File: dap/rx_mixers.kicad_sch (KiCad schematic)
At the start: 2 parts, among them U7 SN74CBT3253, U8 SN74CBT3253

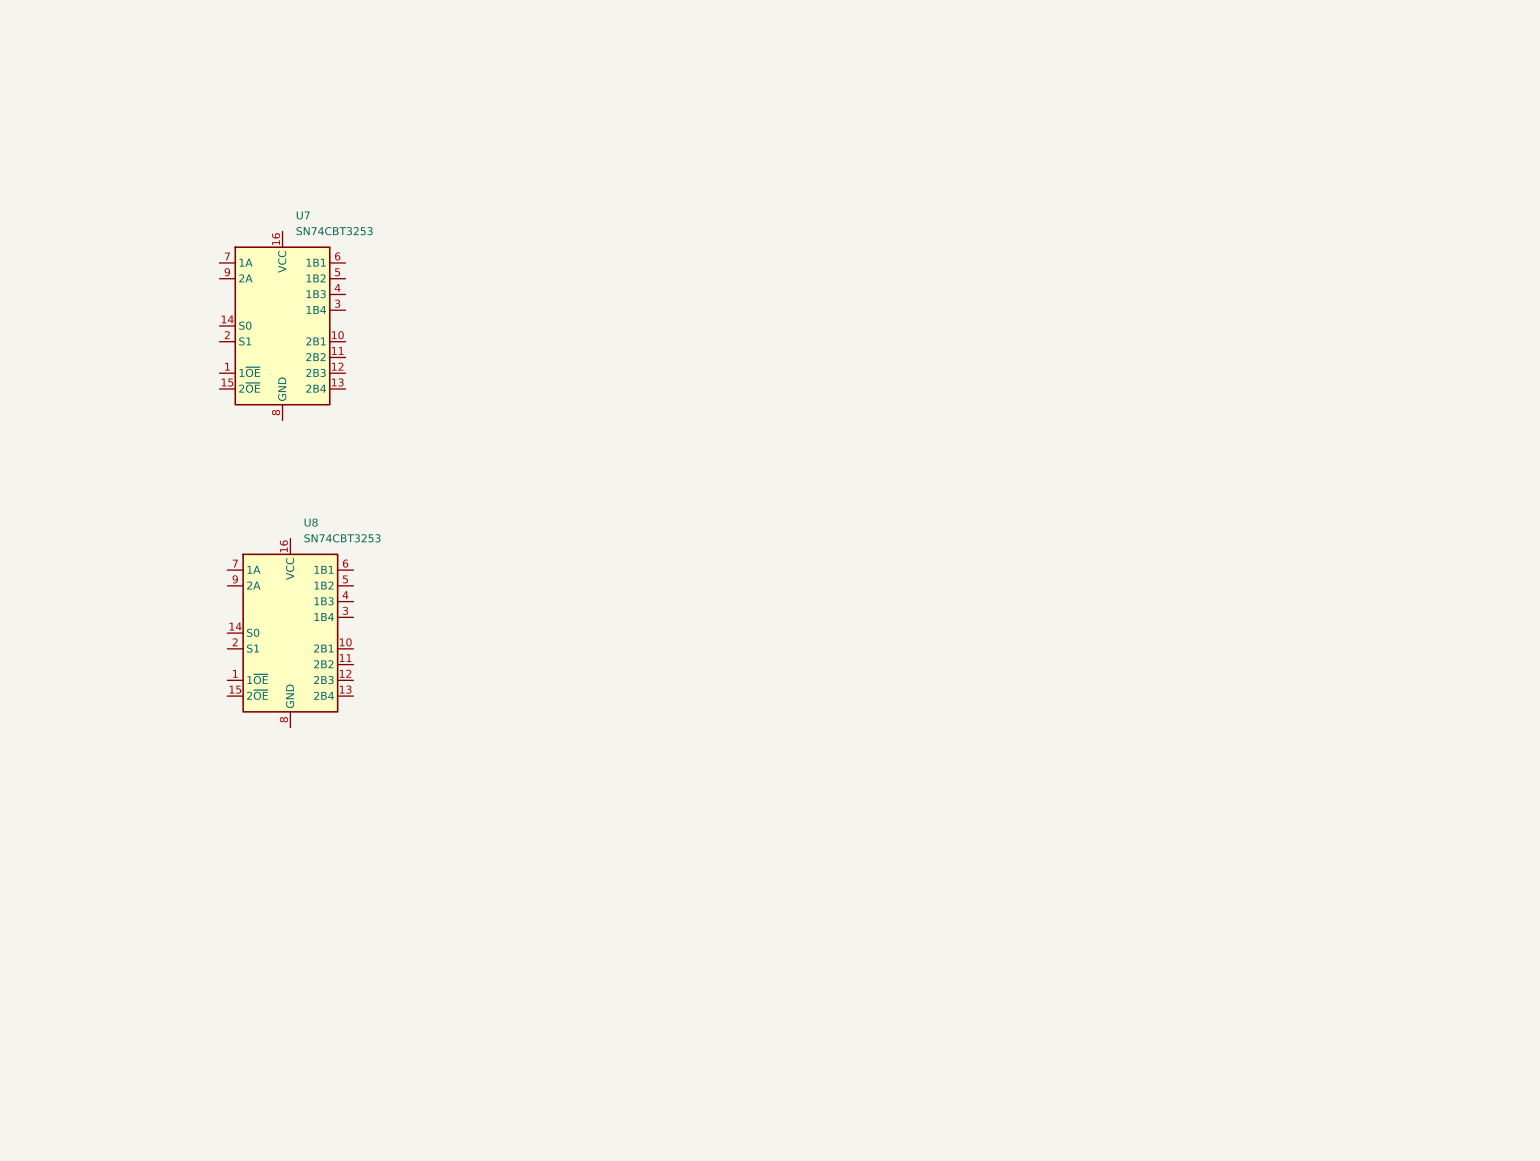
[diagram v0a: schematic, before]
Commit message: general setup
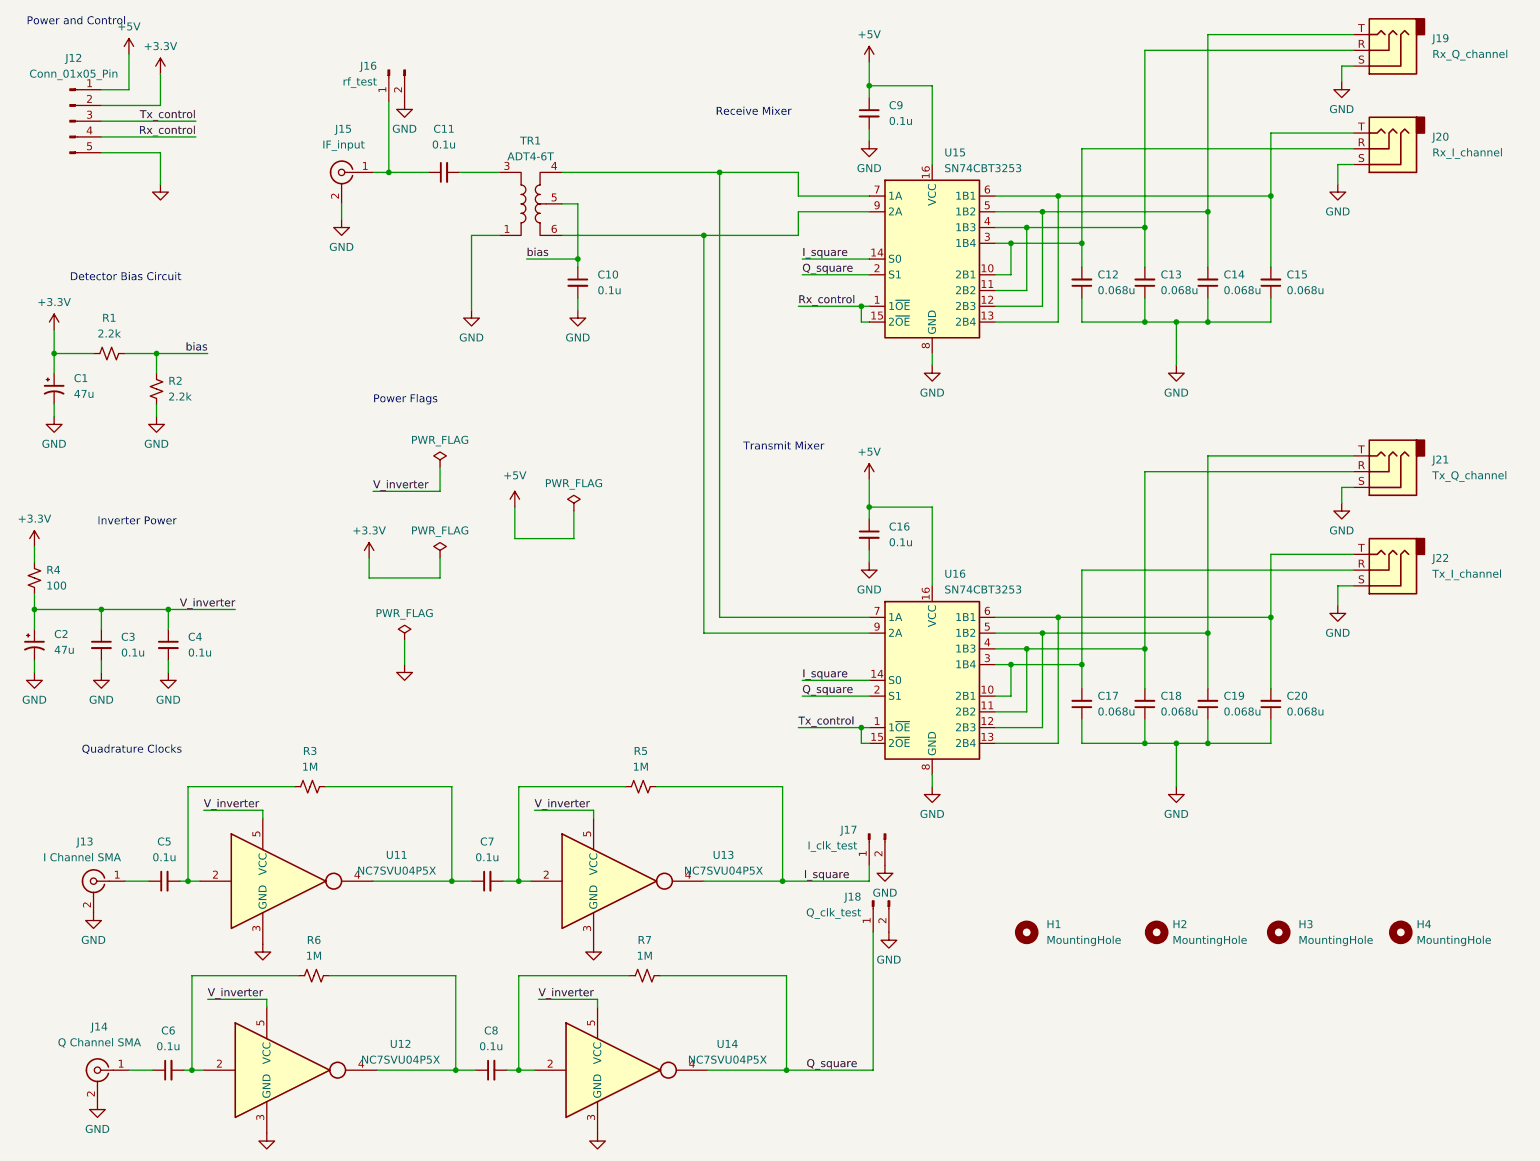
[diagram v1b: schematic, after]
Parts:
- removed U7, U8: SN74CBT3253, symbol Analog_Switch:SN74CBT3253
- added C1, C2: 47u, Capacitor_SMD:C_0805_2012Metric_Pad1.18x1.45mm_HandSolder, symbol Device:C_Polarized_Small_US
- added C10, C11, C16, C3, C4, C5, C6, C7, C8, C9: 0.1u, Capacitor_SMD:C_0805_2012Metric_Pad1.18x1.45mm_HandSolder, symbol Device:C_Small
- added C12, C13, C14, C15, C17, C18, C19, C20: 0.068u, Capacitor_SMD:C_0805_2012Metric_Pad1.18x1.45mm_HandSolder, symbol Device:C_Small
- added H1, H2, H3, H4: MountingHole, MountingHole:MountingHole_3.2mm_M3, symbol Mechanical:MountingHole
- added J12: Conn_01x05_Pin, Connector_PinHeader_2.54mm:PinHeader_1x05_P2.54mm_Vertical, symbol Connector:Conn_01x05_Pin
- added J13: I Channel SMA, Connector_Coaxial:SMA_Amphenol_132289_EdgeMount, symbol Connector:Conn_Coaxial
- added J14: Q Channel SMA, Connector_Coaxial:SMA_Amphenol_132289_EdgeMount, symbol Connector:Conn_Coaxial
- added J15: IF_input, Connector_Coaxial:SMA_Amphenol_132289_EdgeMount, symbol Connector:Conn_Coaxial
- added J16: rf_test, Connector_PinHeader_2.54mm:PinHeader_1x02_P2.54mm_Vertical, symbol Connector:Conn_01x02_Pin
- added J17: I_clk_test, Connector_PinHeader_2.54mm:PinHeader_1x02_P2.54mm_Vertical, symbol Connector:Conn_01x02_Pin
- added J18: Q_clk_test, Connector_PinHeader_2.54mm:PinHeader_1x02_P2.54mm_Vertical, symbol Connector:Conn_01x02_Pin
- added J19: Rx_Q_channel, Connector_Audio:Jack_3.5mm_CUI_SJ-3523-SMT_Horizontal, symbol audiojack3:AudioJack3
- added J20: Rx_I_channel, Connector_Audio:Jack_3.5mm_CUI_SJ-3523-SMT_Horizontal, symbol audiojack3:AudioJack3
- added J21: Tx_Q_channel, Connector_Audio:Jack_3.5mm_CUI_SJ-3523-SMT_Horizontal, symbol audiojack3:AudioJack3
- added J22: Tx_I_channel, Connector_Audio:Jack_3.5mm_CUI_SJ-3523-SMT_Horizontal, symbol audiojack3:AudioJack3
- added R1, R2: 2.2k, Resistor_SMD:R_0805_2012Metric_Pad1.20x1.40mm_HandSolder, symbol Device:R_Small_US
- added R3, R5, R6, R7: 1M, Resistor_SMD:R_0805_2012Metric_Pad1.20x1.40mm_HandSolder, symbol Device:R_Small_US
- added R4: 100, Resistor_SMD:R_0805_2012Metric_Pad1.20x1.40mm_HandSolder, symbol Device:R_Small_US
- added TR1: ADT4-6T, RF_Mini-Circuits:Mini-Circuits_CD637_H5.23mm, symbol Transformer:ADT4-6T
- added U11, U12, U13, U14: NC7SVU04P5X, Package_TO_SOT_SMD:SOT-353_SC-70-5, symbol 74xGxx:NC7SVU04P5X
- added U15, U16: SN74CBT3253, Package_SO:SOIC-16_3.9x9.9mm_P1.27mm, symbol Analog_Switch:SN74CBT3253
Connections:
- new net: C20.2, J22.T, U16.13 (2B4), U16.6 (1B1)
- new net: C12.2, J20.R, U15.10 (2B1), U15.3 (1B4)
- new net: C11.1, J15.1 (In), J16.1 (Pin_1)
- new net: C17.2, J22.R, U16.10 (2B1), U16.3 (1B4)
- new net: C13.2, J19.R, U15.11 (2B2), U15.4 (1B3)
- new net: C14.2, J19.T, U15.12 (2B3), U15.5 (1B2)
- new net: C15.2, J20.T, U15.13 (2B4), U15.6 (1B1)
- new net: TR1.4, U15.7 (1A), U16.7 (1A)
- new net: TR1.6, U15.9 (2A), U16.9 (2A)
- new net: C8.1, R6.1, U12.4
- new net: C6.2, R6.2, U12.2
- new net: C8.2, R7.2, U14.2
- new net: C19.2, J21.T, U16.12 (2B3), U16.5 (1B2)
- new net: C7.1, R3.1, U11.4
- new net: C7.2, R5.2, U13.2
- new net: C5.2, R3.2, U11.2
- new net: C5.1, J13.1 (In)
- new net: C18.2, J21.R, U16.11 (2B2), U16.4 (1B3)
- new net: C11.2, TR1.3
- new net: C6.1, J14.1 (In)
- new net +3.3V: C1.1, J12.2 (Pin_2), R1.1, R4.2
- new net +5V: C16.1, C9.1, J12.1 (Pin_1), U15.16 (VCC), U16.16 (VCC)
- new net GND: C1.2, C10.2, C12.1, C13.1, C14.1, C15.1, C16.2, C17.1, C18.1, C19.1, C2.2, C20.1, C3.2, C4.2, C9.2, J12.5 (Pin_5), J13.2 (Ext), J14.2 (Ext), J15.2 (Ext), J16.2 (Pin_2), J17.2 (Pin_2), J18.2 (Pin_2), J19.S, J20.S, J21.S, J22.S, R2.1, TR1.1, U11.3 (GND), U12.3 (GND), U13.3 (GND), U14.3 (GND), U15.8 (GND), U16.8 (GND)
- new net I_square: J17.1 (Pin_1), R5.1, U13.4, U15.14 (S0), U16.14 (S0)
- new net Q_square: J18.1 (Pin_1), R7.1, U14.4, U15.2 (S1), U16.2 (S1)
- new net Rx_control: J12.4 (Pin_4), U15.1 (1~{OE}), U15.15 (2~{OE})
- new net Tx_control: J12.3 (Pin_3), U16.1 (1~{OE}), U16.15 (2~{OE})
- new net V_inverter: C2.1, C3.1, C4.1, R4.1, U11.5 (VCC), U12.5 (VCC), U13.5 (VCC), U14.5 (VCC)
- new net bias: C10.1, R1.2, R2.2, TR1.5
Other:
- note added: "Detector Bias Circuit"
- note added: "Inverter Power"
- note added: "Power Flags"
- note added: "Power and Control"
- note added: "Quadrature Clocks"
- note added: "Receive Mixer"
- note added: "Transmit Mixer"
